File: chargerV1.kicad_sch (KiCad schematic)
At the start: 46 parts, among them J1 USB_C_Receptacle, J2 SOCKET_1x4, J3 SOCKET_1x4, J4 SOCKET_1x6, J5 Micro_SD_Card, SW1 BOOT, SW2 OK, SW3 RESET, SW4 UP, SW5 DW, U1 DS3231M, U2 ESP32-WROOM-32D, U4 AMS1117-3.3

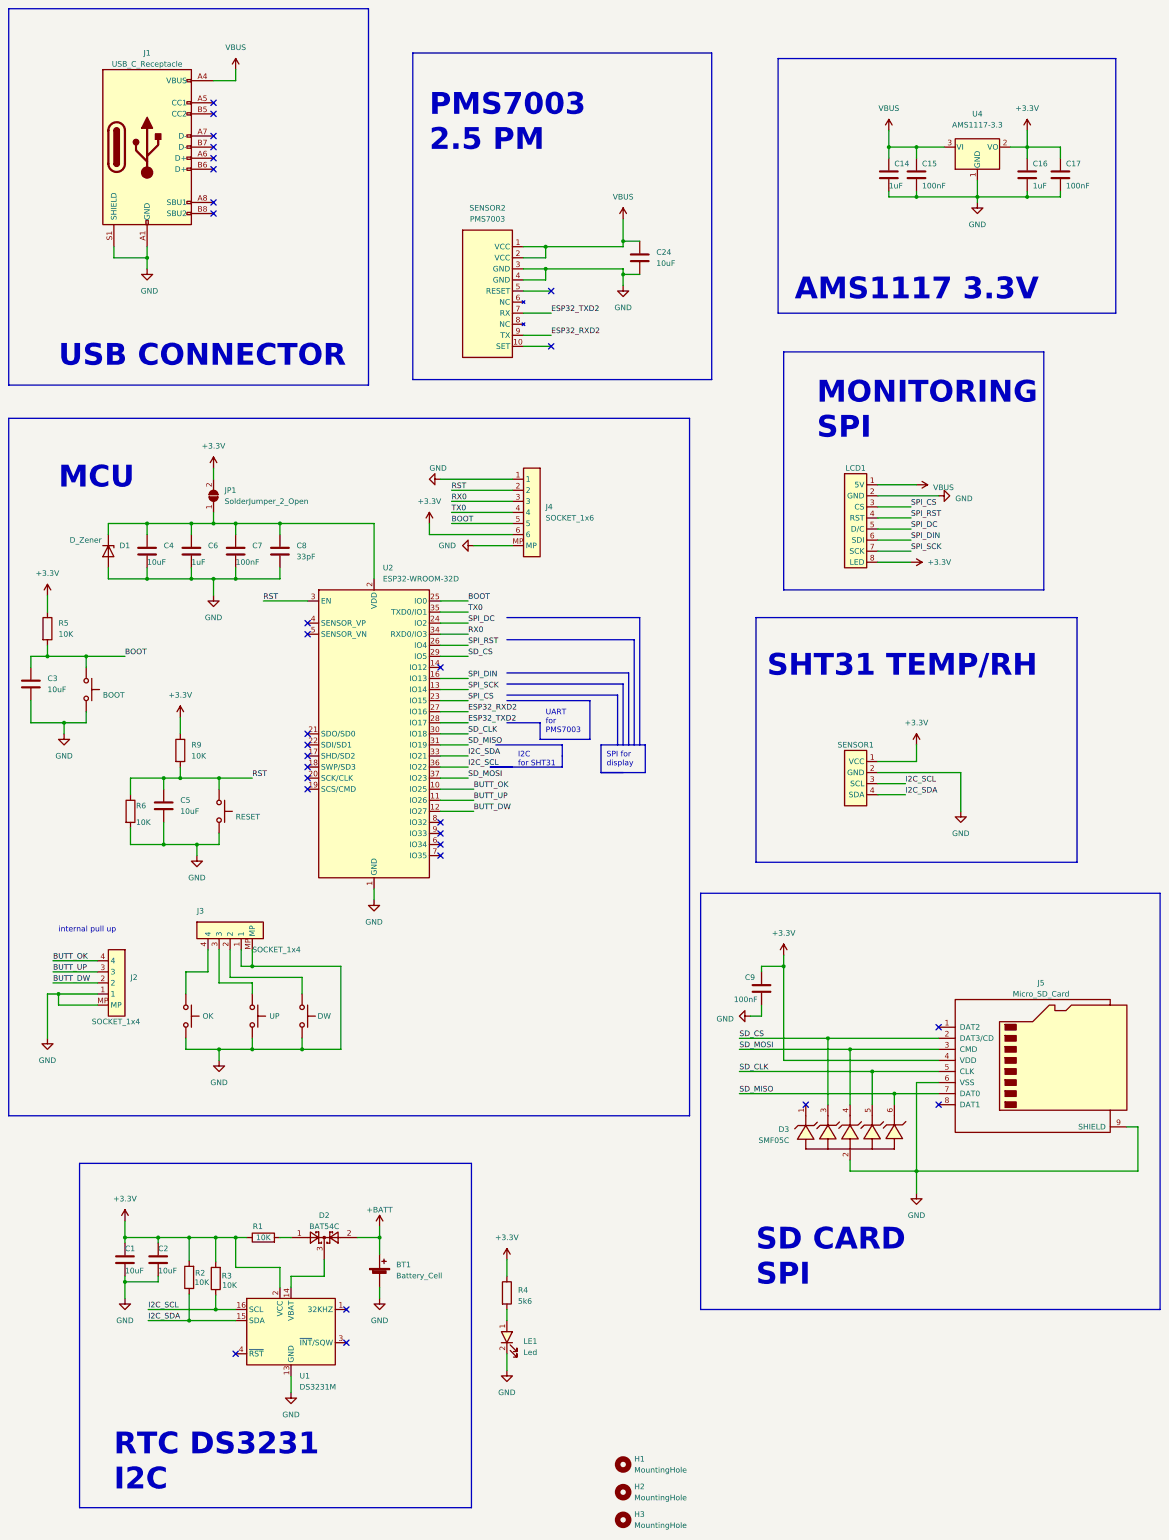
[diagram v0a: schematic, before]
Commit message: Add modifies
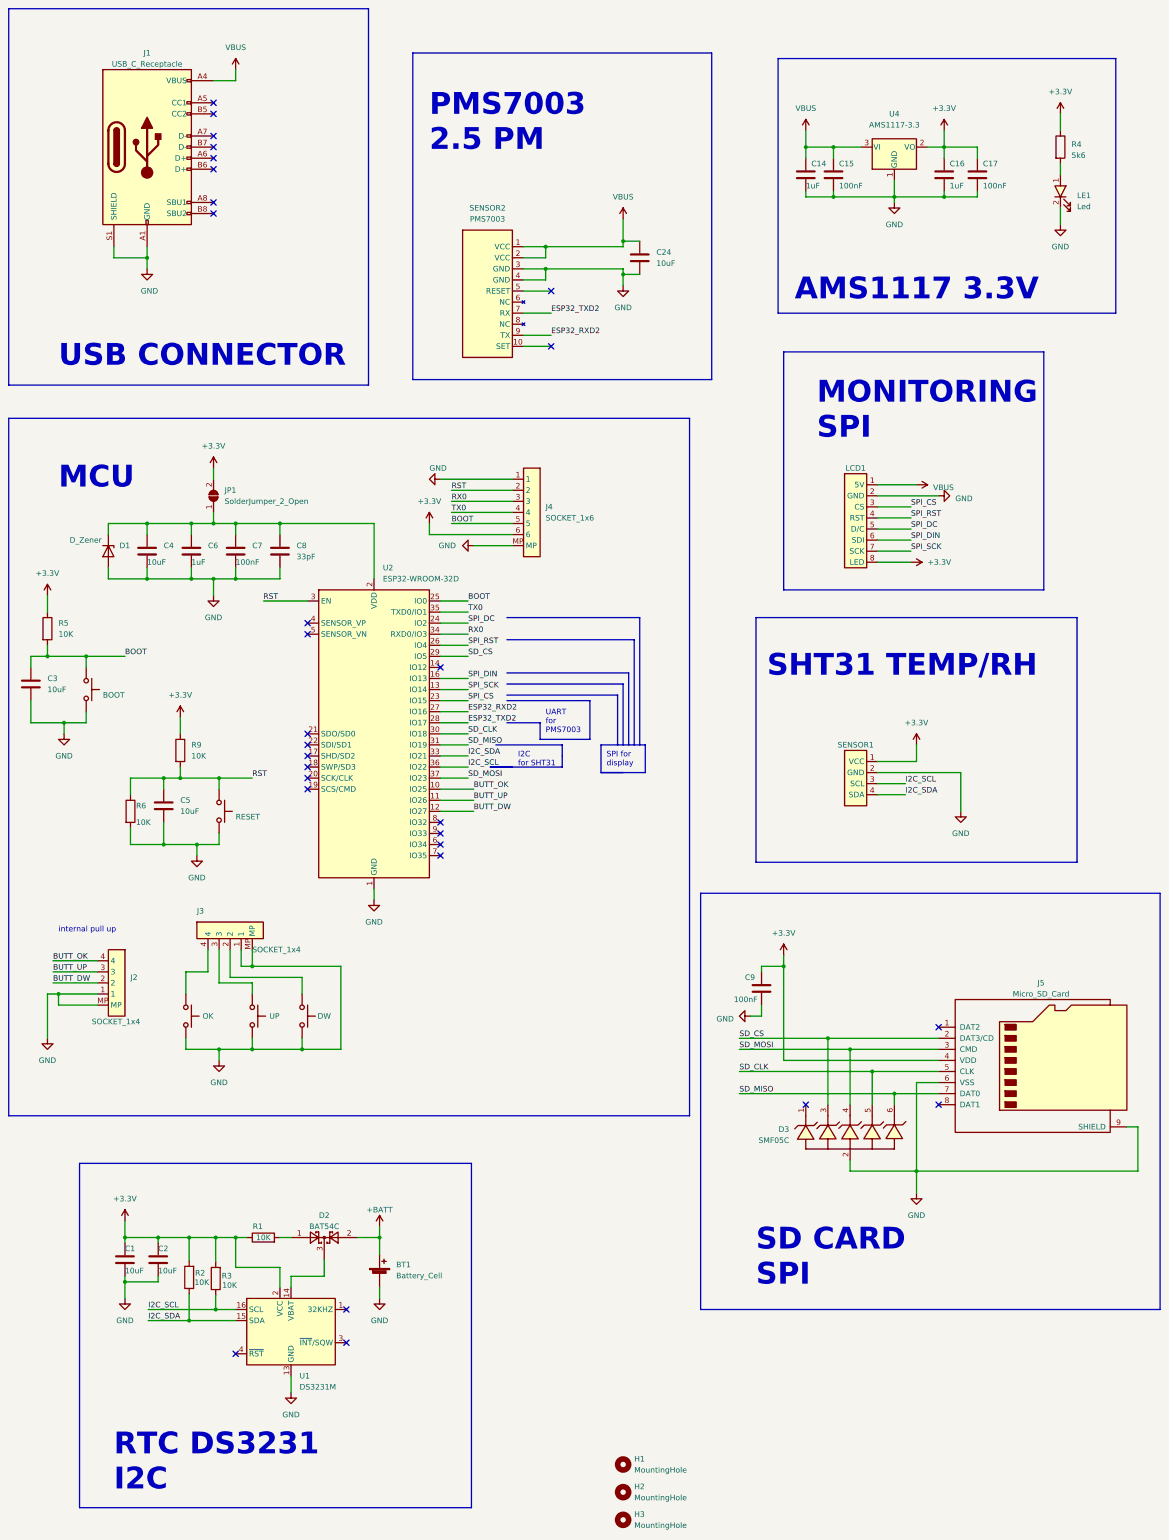
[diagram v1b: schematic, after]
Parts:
- C14, C15, C16, C17, C24: footprint IVSFootprint:C0603 -> IVS_footprints:C_0603
- J2, J3, SENSOR1: footprint IVSFootprint:SH-1.0mm-1x4 -> IVS_footprints:JST_SH_SM04B-SRSS-TB_1x04-1MP_P1.00mm_Horizontal
- J4: footprint IVSFootprint:SH-1.0mm-1x6 -> IVS_footprints:JST_SH_SM06B-SRSS-TB_1x06-1MP_P1.00mm_Horizontal
- LCD1: footprint IVSFootprint:SH-1.0mm-1x8 -> IVS_footprints:JST_SH_SM08B-SRSS-TB_1x08-1MP_P1.00mm_Horizontal
- SW1, SW3: footprint IVSFootprint:SW_SPST_PTS810 -> IVS_footprints:SW_SPST_PTS810
- SW2, SW4, SW5: footprint IVS_footprints:BUTTON_PUSH_12mm -> IVS_footprints:Button_Push_12mm
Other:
- moved on the sheet: C14, C15, C16, C17, LE1, R4, U4

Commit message: Add more modifies
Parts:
- C4, C6, C7, C8: footprint IVSFootprint:C0603 -> IVS_footprints:C_0603
- D1: footprint IVSFootprint:D_MiniMELF -> IVS_footprints:D_MiniMELF
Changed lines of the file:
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@@
       (effects (font (size 1.27 1.27)) (justify left))
     )
-    (property "Footprint" "IVSFootprint:C0603" (at 60.6552 175.26 0)
+    (property "Footprint" "IVS_footprints:C_0603" (at 60.6552 175.26 0)
       (effects (font (size 1.27 1.27)) hide)
     )
@@
       (effects (font (size 1.27 1.27)) (justify left))
     )
-    (property "Footprint" "IVSFootprint:C0603" (at 50.4952 175.26 0)
+    (property "Footprint" "IVS_footprints:C_0603" (at 50.4952 175.26 0)
       (effects (font (size 1.27 1.27)) hide)
     )
@@
       (effects (font (size 1.27 1.27)) (justify left))
     )
-    (property "Footprint" "IVSFootprint:C0603" (at 80.9752 175.26 0)
+    (property "Footprint" "IVS_footprints:C_0603" (at 80.9752 175.26 0)
       (effects (font (size 1.27 1.27)) hide)
     )
@@
       (effects (font (size 1.27 1.27)) (justify left))
     )
-    (property "Footprint" "IVSFootprint:D_MiniMELF" (at 40.64 171.45 0)
+    (property "Footprint" "IVS_footprints:D_MiniMELF" (at 40.64 171.45 0)
       (effects (font (size 1.27 1.27)) hide)
     )
@@
       (effects (font (size 1.27 1.27)) (justify left))
     )
-    (property "Footprint" "IVSFootprint:C0603" (at 70.8152 175.26 0)
-      (effects (font (size 1.27 1.27)) hide)
-    )
+    (property "Footprint" "IVS_footprints:C_0603" (at 70.8152 175.26 0)
+      (effects (font (size 1.27 1.27)) hide)
+    )
